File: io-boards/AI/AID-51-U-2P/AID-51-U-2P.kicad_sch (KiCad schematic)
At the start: 0 parts

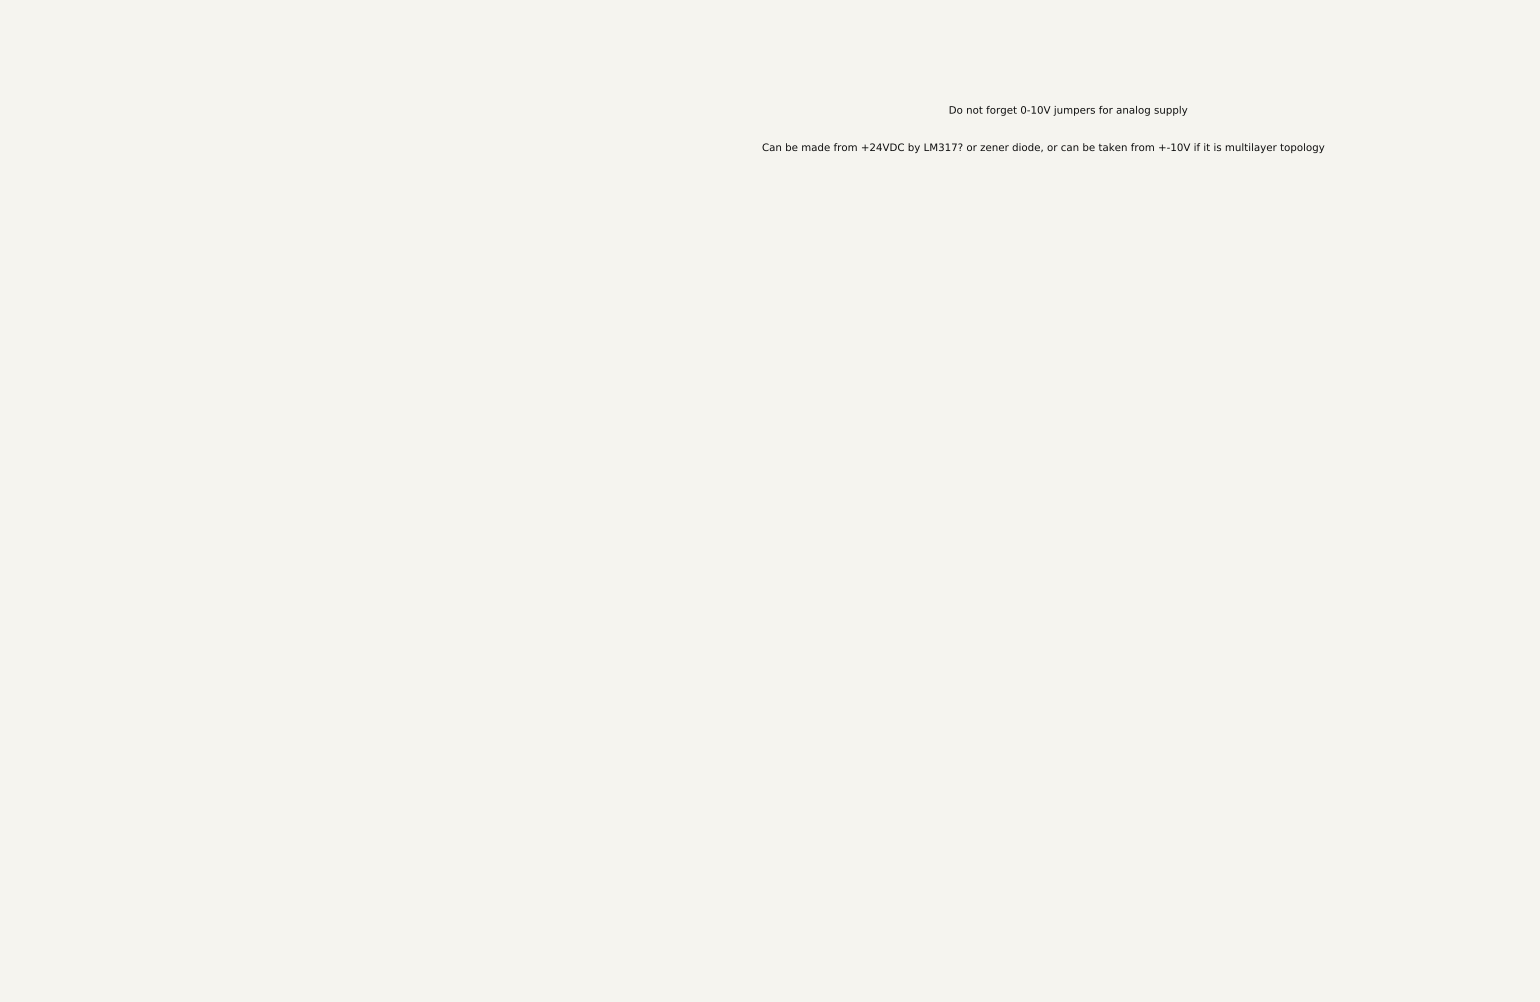
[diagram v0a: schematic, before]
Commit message: AI board has been finnished.
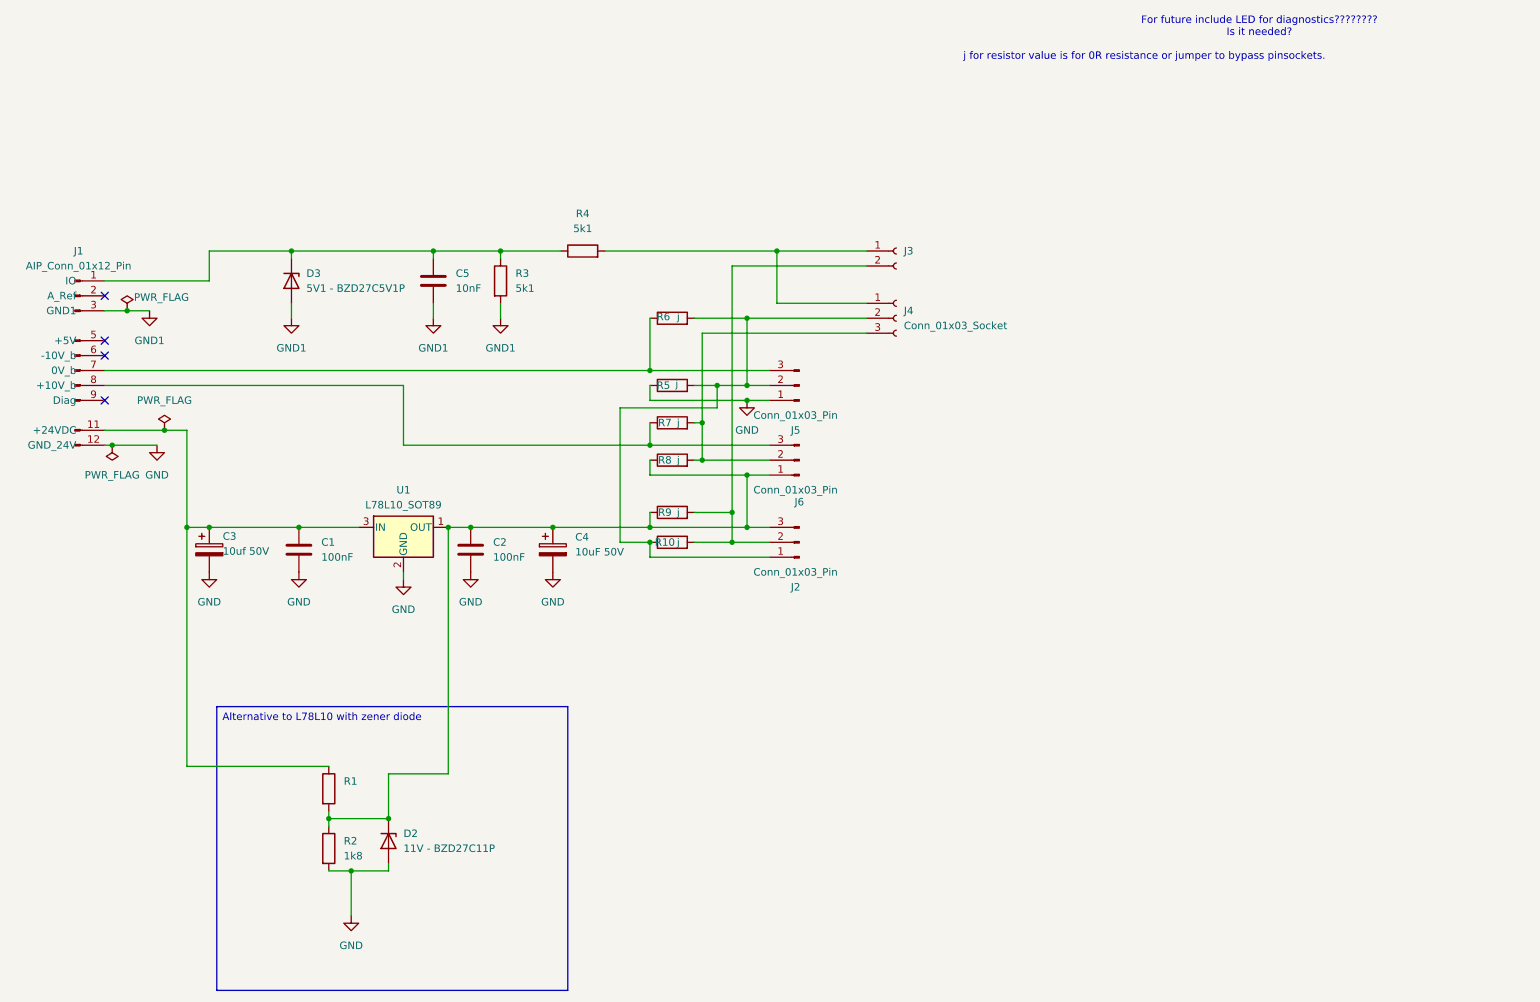
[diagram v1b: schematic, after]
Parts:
- added C1, C2: 100nF, Capacitor_SMD:C_0402_1005Metric, symbol Device:C
- added C3: 10uf 50V, Capacitor_SMD:CP_Elec_3x5.3, symbol Device:C_Polarized
- added C4: 10uF 50V, Capacitor_SMD:CP_Elec_3x5.3, symbol Device:C_Polarized
- added C5: 10nF, Capacitor_SMD:C_0402_1005Metric, symbol Device:C
- added D2: 11V - BZD27C11P, Diode_SMD:D_SMF, symbol Diode:BZD27Cxx
- added D3: 5V1 - BZD27C5V1P, Diode_SMD:D_SMF, symbol Diode:BZD27Cxx
- added J1: AIP_Conn_01x12_Pin, tuxmio:IO_AIP_PinHeader_1x12_P2.54mm_Horizontal, symbol tuxmio:IO_AIP_Conn_01x12_Pin
- added J2, J5, J6: Conn_01x03_Pin, Connector_PinHeader_2.54mm:PinHeader_1x03_P2.54mm_Horizontal, symbol Connector:Conn_01x03_Pin
- added J3: Conn_01x02_Socket, tuxmio:KF141x_SMD, symbol Connector:Conn_01x02_Socket
- added J4: Conn_01x03_Socket, Connector_PinSocket_2.54mm:PinSocket_1x03_P2.54mm_Horizontal, symbol Connector:Conn_01x03_Socket
- added R1: 2k2, Resistor_SMD:R_0402_1005Metric_Pad0.72x0.64mm_HandSolder, symbol Device:R
- added R10, R5, R6, R7, R8, R9: j, Resistor_SMD:R_0201_0603Metric, symbol Device:R
- added R2: 1k8, Resistor_SMD:R_0402_1005Metric_Pad0.72x0.64mm_HandSolder, symbol Device:R
- added R3, R4: 5k1, Resistor_SMD:R_0402_1005Metric_Pad0.72x0.64mm_HandSolder, symbol Device:R
- added U1: L78L10_SOT89, Package_TO_SOT_SMD:SOT-89-3, symbol Regulator_Linear:L78L10_SOT89
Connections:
- new net: C1.1, C3.1, J1.11 (+24VDC), R1.1, U1.3 (IN)
- new net: C2.1, C4.1, D2.1 (K), J2.3 (Pin_3), J6.1 (Pin_1), R1.2, R2.1, R8.1, R9.1, U1.1 (OUT)
- new net: J1.8 (+10V_b), J6.3 (Pin_3), R7.1
- new net: J4.3 (Pin_3), J6.2 (Pin_2), R7.2, R8.2
- new net: J2.1 (Pin_1), J4.2 (Pin_2), J5.2 (Pin_2), R10.1, R5.2, R6.2
- new net: J1.7 (0V_b), J5.3 (Pin_3), R6.1
- new net: C5.1, D3.1 (K), J1.1 (IO), R3.1, R4.1
- new net: J2.2 (Pin_2), J3.2 (Pin_2), R10.2, R9.2
- new net: J3.1 (Pin_1), J4.1 (Pin_1), R4.2
- new net GND: C1.2, C2.2, C3.2, C4.2, D2.2 (A), J1.12 (GND_24V), J5.1 (Pin_1), R2.2, R5.1, U1.2 (GND)
- new net GND1: C5.2, D3.2 (A), J1.3 (GND1), R3.2
- no-connect marks 0 -> 4
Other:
- note added: "For future include LED for diagnostics???????? Is it needed?"
- note added: "j for resistor value is for 0R resistance or jumper to bypass pinsockets."
